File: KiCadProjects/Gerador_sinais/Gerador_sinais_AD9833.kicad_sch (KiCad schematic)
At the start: 17 parts, among them J1 tensoes, J3 sinais analogicos, J4 comunicacao / sinais digitais, J6 pinos de prova, SW1 botao_forma_onda, SW2 botao_incremento_freq, SW3 botao_decremento_freq, SW4 botao_save_Rgain, SW5 botao_aumenta_Rgain, SW6 botao_diminui_Rgain, U1 AD828AN, U2 X9c10x, U3 AD9833_module

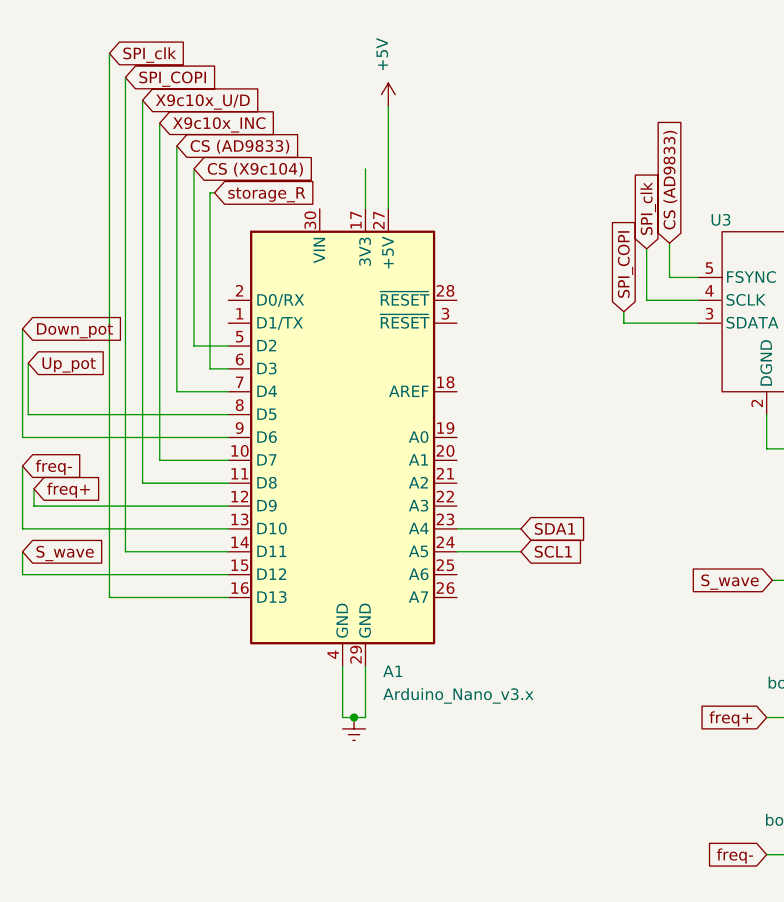
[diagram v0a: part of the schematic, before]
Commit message: Atribuição dos footprints
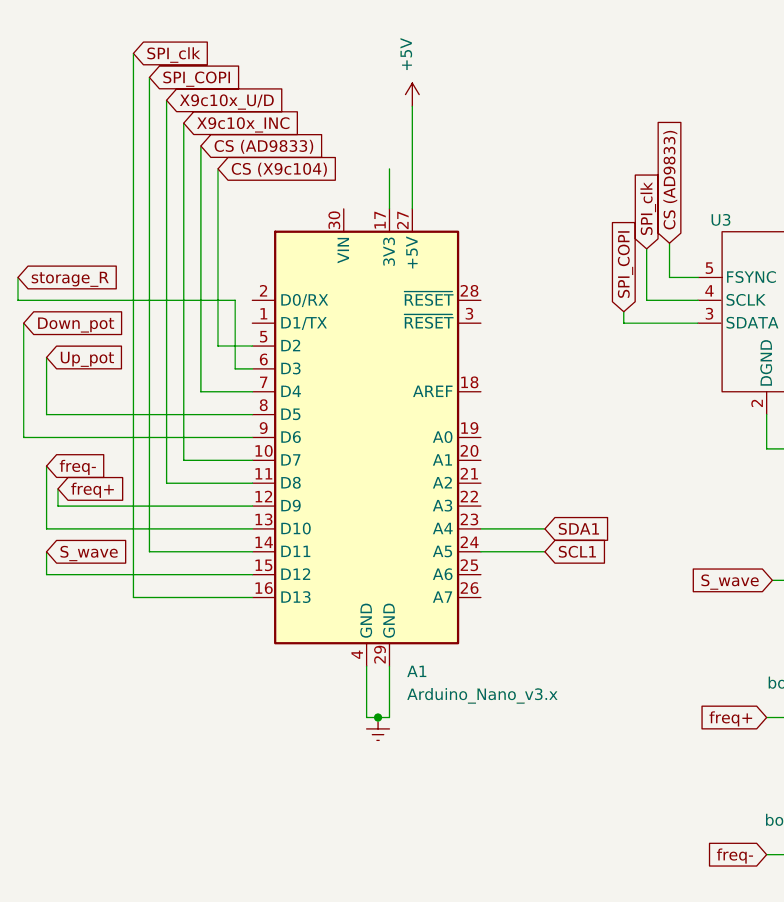
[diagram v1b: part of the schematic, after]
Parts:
- U1: footprint footprints:N_8_ADI -> AD828AN:N_8_ADI
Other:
- moved on the sheet: A1

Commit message: Atribuição dos footprints
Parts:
- U1: footprint AD828AN:N_8_ADI -> AD828:N_8_ADI
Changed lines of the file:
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@@
       (effects (font (size 1.524 1.524)))
     )
-    (property "Footprint" "AD828AN:N_8_ADI" (at 177.165 45.085 0)
+    (property "Footprint" "AD828:N_8_ADI" (at 177.165 45.085 0)
       (effects (font (size 1.27 1.27) italic) hide)
     )
